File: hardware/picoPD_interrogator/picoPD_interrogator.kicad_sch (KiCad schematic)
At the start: 54 parts, among them J1 Conn_01x07, J2 USB_C_Receptacle_USB2.0_16P, J3 Conn_01x14, Q1 rohm-RE1C002UN, Q2 rohm-RE1C002UN, Q3 rohm-RE1C002UN, Q4 rohm-RE1C002UN, Q5 rohm-RE1C002UN, SW1 RESET_BTN, U3 ST-LM393QT, U6 LV2862XDDC

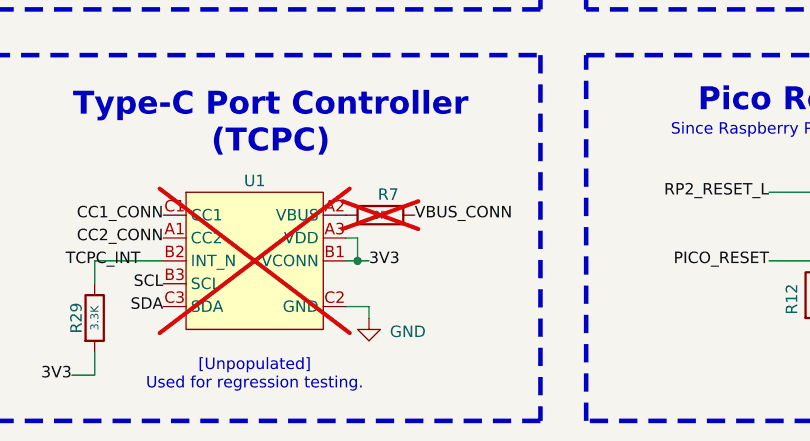
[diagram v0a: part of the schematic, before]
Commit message: PCB: Working on PCB layout.
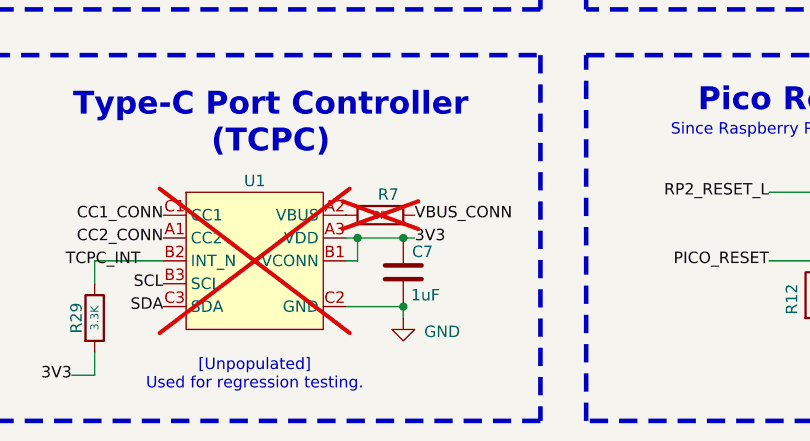
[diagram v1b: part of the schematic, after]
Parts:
- added C7: 1uF, Capacitor_SMD:C_0603_1608Metric, symbol Device:C
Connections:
- net 3V3: now also C7.2
- net GND: now also C7.1
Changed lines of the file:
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@@
 	)
 	(junction
+		(at 62.23 180.34)
+		(diameter 0)
+		(color 0 0 0 0)
+	)
+	(junction
 		(at 114.3 184.15)
 		(diameter 0)
@@
 	)
 	(junction
+		(at 57.15 172.72)
+		(diameter 0)
+		(color 0 0 0 0)
+	)
+	(junction
 		(at 143.51 116.84)
 		(diameter 0)
@@
 	)
 	(junction
-		(at 57.15 175.26)
+		(at 62.23 172.72)
 		(diameter 0)
 		(color 0 0 0 0)
@@
 	(wire
 		(pts
+			(xy 62.23 172.72) (xy 63.5 172.72)
+		)
+		(stroke
+			(width 0)
+			(type default)
+		)
+	)
+	(wire
+		(pts
 			(xy 102.87 54.61) (xy 102.87 55.88)
 		)
@@
 	(wire
 		(pts
+			(xy 57.15 172.72) (xy 62.23 172.72)
+		)
+		(stroke
+			(width 0)
+			(type default)
+		)
+	)
+	(wire
+		(pts
 			(xy 237.49 106.68) (xy 240.03 106.68)
 		)
@@
 	(wire
 		(pts
-			(xy 57.15 175.26) (xy 58.42 175.26)
-		)
-		(stroke
-			(width 0)
-			(type default)
-		)
-	)
-	(wire
-		(pts
 			(xy 63.5 78.74) (xy 66.04 78.74)
 		)
@@
 	(wire
 		(pts
-			(xy 57.15 172.72) (xy 57.15 175.26)
-		)
-		(stroke
-			(width 0)
-			(type default)
-		)
-	)
-	(wire
-		(pts
 			(xy 102.87 55.88) (xy 102.87 57.15)
 		)
@@
 	(wire
 		(pts
-			(xy 55.88 180.34) (xy 58.42 180.34)
+			(xy 55.88 180.34) (xy 62.23 180.34)
 		)
 		(stroke
@@
 	(wire
 		(pts
-			(xy 58.42 180.34) (xy 58.42 181.61)
-		)
-		(stroke
-			(width 0)
-			(type default)
-		)
-	)
-	(wire
-		(pts
 			(xy 170.18 39.37) (xy 170.18 53.34)
 		)
@@
 	(wire
 		(pts
+			(xy 57.15 172.72) (xy 57.15 175.26)
+		)
+		(stroke
+			(width 0)
+			(type default)
+		)
+	)
+	(wire
+		(pts
+			(xy 62.23 180.34) (xy 62.23 181.61)
+		)
+		(stroke
+			(width 0)
+			(type default)
+		)
+	)
+	(wire
+		(pts
 			(xy 269.24 132.08) (xy 270.51 132.08)
 		)
@@
 	)
 	(label "3V3"
-		(at 58.42 175.26 0)
+		(at 63.5 172.72 0)
 		(effects
 			(font
@@
 	(symbol
 		(lib_id "power:GND")
-		(at 58.42 181.61 0)
+		(at 62.23 181.61 0)
 		(mirror y)
 		(unit 1)
@@
 		(dnp no)
 		(property "Reference" "#PWR06"
-			(at 58.42 187.96 0)
+			(at 62.23 187.96 0)
 			(effects
 				(font
@@
 		)
 		(property "Value" "GND"
-			(at 62.738 183.134 0)
+			(at 66.548 183.134 0)
 			(effects
 				(font
@@
 		)
 		(property "Footprint" ""
-			(at 58.42 181.61 0)
+			(at 62.23 181.61 0)
 			(effects
 				(font
@@
 		)
 		(property "Datasheet" ""
-			(at 58.42 181.61 0)
+			(at 62.23 181.61 0)
 			(effects
 				(font
@@
 		)
 		(property "Description" "Power symbol creates a global label with name \"GND\" , ground"
-			(at 58.42 181.61 0)
+			(at 62.23 181.61 0)
 			(effects
 				(font
@@
 					(unit 1)
 				)
+			)
+		)
+	)
+	(symbol
+		(lib_id "Device:C")
+		(at 62.23 176.53 180)
+		(unit 1)
+		(exclude_from_sim no)
+		(in_bom yes)
+		(on_board yes)
+		(dnp no)
+		(property "Reference" "C7"
+			(at 65.532 174.244 0)
+			(effects
+				(font
+					(size 1.27 1.27)
+				)
+				(justify left)
+			)
+		)
+		(property "Value" "1uF"
+			(at 66.294 179.07 0)
+			(effects
+				(font
+					(size 1.27 1.27)
+				)
+				(justify left)
+			)
+		)
+		(property "Footprint" "Capacitor_SMD:C_0603_1608Metric"
+			(at 61.2648 172.72 0)
+			(effects
+				(font
+					(size 1.27 1.27)
+				)
+				(hide yes)
+			)
+		)
+		(property "Datasheet" "~"
+			(at 62.23 176.53 0)
+			(effects
+				(font
+					(size 1.27 1.27)
+				)
+				(hide yes)
+			)
+		)
+		(property "Description" "Unpolarized capacitor"
+			(at 62.23 176.53 0)
+			(effects
+				(font
+					(size 1.27 1.27)
+				)
+				(hide yes)
+			)
+		)
+		(property "Description Detailed" "1 µF ±10% 50V Ceramic Capacitor X5R 0603 (1608 Metric)"
+			(at 62.23 176.53 0)
+			(effects
+				(font
+					(size 1.27 1.27)
+				)
+				(hide yes)
+			)
+		)
+		(property "Manufacturer PN" "GRT188R61H105KE13D"
+			(at 62.23 176.53 0)
+			(effects
+				(font
+					(size 1.27 1.27)
+				)
+				(hide yes)
+			)
+		)
+		(property "Manufacturer" "Murata Electronics"
+			(at 62.23 176.53 0)
+			(effects
+				(font
+					(size 1.27 1.27)
+				)
+				(hide yes)
+			)
+		)
+		(property "DigiKey PN" "490-12330-1-ND"
+			(at 62.23 176.53 0)
+			(effects
+				(font
+					(size 1.27 1.27)
+				)
+				(hide yes)
+			)
+		)
+		(pin "2"
+		)
+		(pin "1"
+		)
+		(instances
+			(project "picoPD_interrogator"
+				(path "/e34b0978-7def-4921-94d0-accc0a677529"
+					(reference "C7")
+					(unit 1)
+				)
